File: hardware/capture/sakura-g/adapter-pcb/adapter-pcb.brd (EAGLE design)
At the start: 55.9 x 22.5 mm, 6 parts

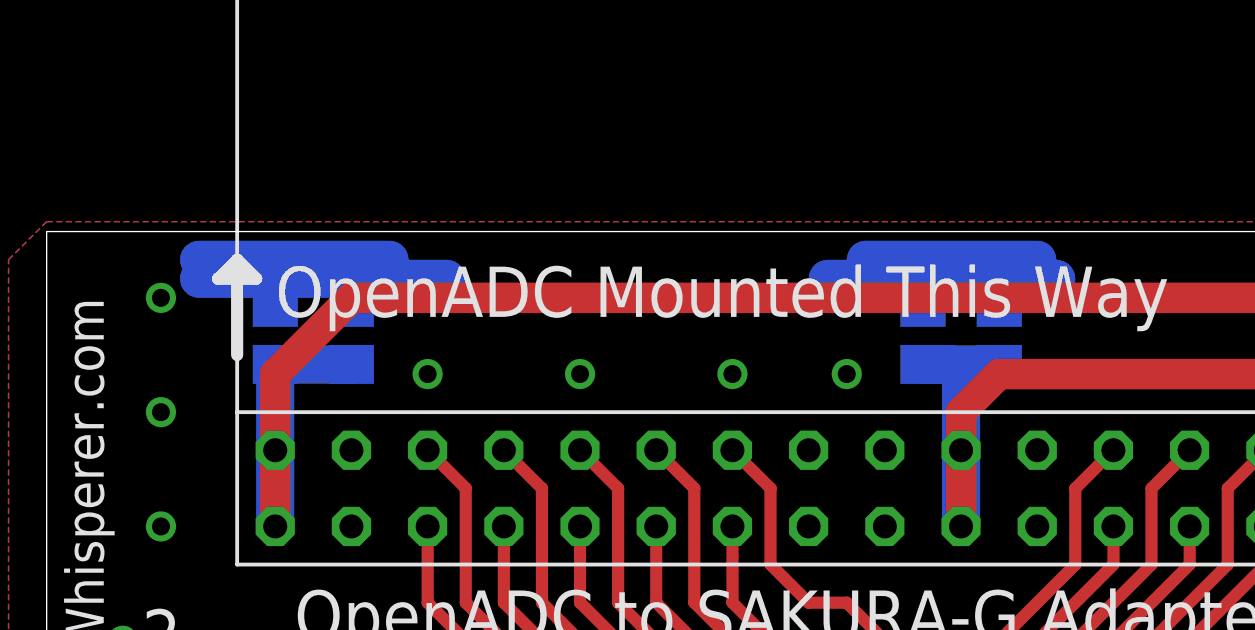
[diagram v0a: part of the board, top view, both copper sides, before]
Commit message: Updates to PCBs, add new PCBs
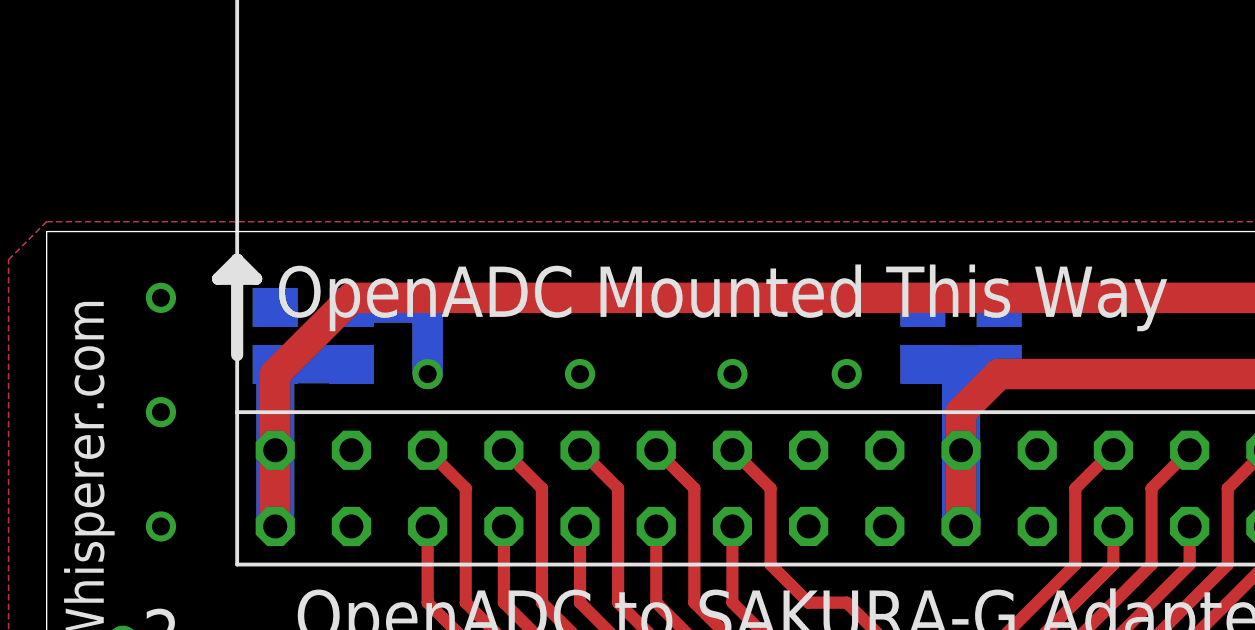
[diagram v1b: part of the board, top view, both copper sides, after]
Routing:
- net N$5: track 8.25 -> 0.00 mm
- net N$6: track 7.62 -> 0.00 mm
- net N$8: track 6.35 -> 0.00 mm
- net N$7: track 5.72 -> 0.00 mm
- net GND: track 1.80 -> 6.37 mm
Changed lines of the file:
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@@
 <?xml version="1.0" encoding="utf-8"?>
 <!DOCTYPE eagle SYSTEM "eagle.dtd">
-<eagle version="6.4">
+<eagle version="6.5.0">
 <drawing>
 <settings>
@@
 <setting verticaltext="up"/>
 </settings>
-<grid distance="0.025" unitdist="inch" unit="inch" style="lines" multiple="1" display="no" altdistance="0.025" altunitdist="inch" altunit="inch"/>
+<grid distance="0.025" unitdist="inch" unit="mm" style="lines" multiple="1" display="no" altdistance="0.025" altunitdist="inch" altunit="inch"/>
 <layers>
 <layer number="1" name="Top" color="4" fill="1" visible="yes" active="yes"/>
@@
 <via x="22.86" y="17.78" extent="1-16" drill="0.6" shape="octagon"/>
 <via x="17.78" y="17.78" extent="1-16" drill="0.6" shape="octagon"/>
+<wire x1="15.24" y1="20" x2="17.465" y2="20" width="1.016" layer="16"/>
+<wire x1="17.465" y1="20" x2="17.78" y2="19.685" width="1.016" layer="16"/>
+<wire x1="17.78" y1="19.685" x2="17.78" y2="17.78" width="1.016" layer="16"/>
 </signal>
 <signal name="N$1">
@@
 <wire x1="29.21" y1="13.97" x2="27.94" y2="15.24" width="0.4064" layer="1"/>
 </signal>
-<signal name="N$5">
-<wire x1="10.16" y1="20.955" x2="18.415" y2="20.955" width="1.27" layer="16"/>
-</signal>
-<signal name="N$6">
-<wire x1="31.115" y1="20.955" x2="38.735" y2="20.955" width="1.27" layer="16"/>
-</signal>
-<signal name="N$7">
-<wire x1="32.385" y1="21.59" x2="38.1" y2="21.59" width="1.27" layer="16"/>
-</signal>
-<signal name="N$8">
-<wire x1="10.16" y1="21.59" x2="16.51" y2="21.59" width="1.27" layer="16"/>
-</signal>
 </signals>
